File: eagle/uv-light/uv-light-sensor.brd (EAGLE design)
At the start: 17 x 13 mm, 4 parts, among them IC100 SI1147

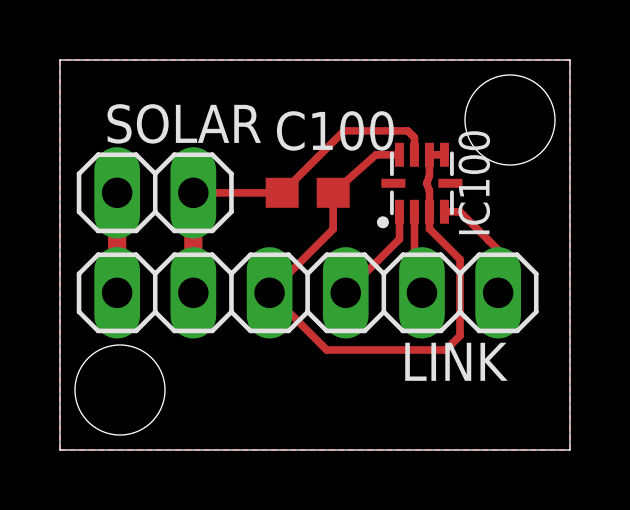
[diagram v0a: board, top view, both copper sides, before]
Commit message: CHG: updated lib, schematics and boards
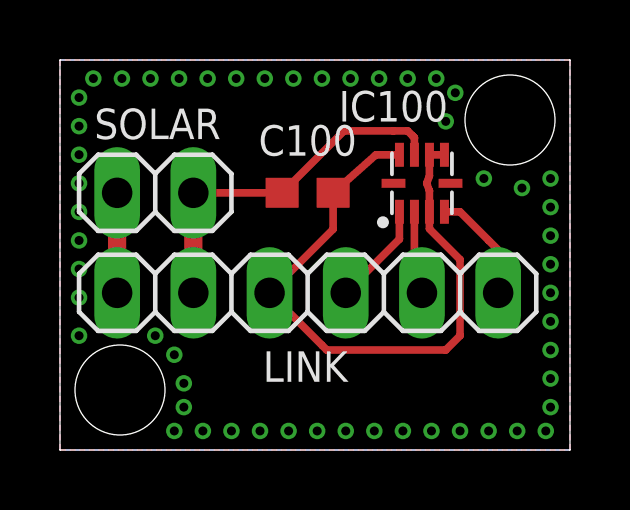
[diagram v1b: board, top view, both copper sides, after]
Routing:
- net GND: vias 0 -> 53
- added copper zone on layer 16, net GND
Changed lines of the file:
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@@
 <element name="IC100" library="weather_station" package="QFN-10/2MM" value="SI1147" x="12.065" y="8.89" smashed="yes" rot="R90">
 <attribute name="DIGIKEY" value="336-2624-1-ND" x="26.035" y="24.13" size="1.778" layer="27" rot="R90" display="off"/>
-<attribute name="NAME" x="14.31625" y="8.89" size="1.016" layer="25" font="vector" ratio="12" rot="R90" align="bottom-center"/>
+<attribute name="NAME" x="11.1125" y="11.45875" size="1.016" layer="25" font="vector" ratio="12" rot="R180" align="center"/>
 </element>
 <element name="C100" library="rcl" package="C0603" value="100n" x="8.255" y="8.5725" smashed="yes">
-<attribute name="NAME" x="7.14375" y="10.00125" size="1.27" layer="25"/>
+<attribute name="NAME" x="8.255" y="10.31875" size="1.016" layer="25" align="center"/>
 <attribute name="VALUE" x="7.62" y="6.6675" size="1.27" layer="27"/>
 </element>
 <element name="LINK" library="pinhead" package="1X06" value="" x="8.255" y="5.23875" smashed="yes">
-<attribute name="NAME" x="11.3538" y="2.30505" size="1.27" layer="25" ratio="10"/>
+<attribute name="NAME" x="8.1788" y="2.7813" size="1.016" layer="25" ratio="10" align="center"/>
 <attribute name="VALUE" x="0.635" y="2.06375" size="1.27" layer="27"/>
 </element>
 <element name="SOLAR" library="pinhead" package="1X02" value="" x="3.175" y="8.5725" smashed="yes" rot="R180">
-<attribute name="NAME" x="6.7437" y="11.5062" size="1.27" layer="25" ratio="10" rot="R180"/>
+<attribute name="NAME" x="3.2512" y="10.8712" size="1.016" layer="25" ratio="10" rot="R180" align="center"/>
 <attribute name="VALUE" x="5.715" y="11.7475" size="1.27" layer="27" rot="R180"/>
 </element>
@@
 <wire x1="11.7475" y1="10.4775" x2="11.815" y2="10.41" width="0.254" layer="1"/>
 <wire x1="11.815" y1="10.41" x2="11.815" y2="9.84" width="0.254" layer="1"/>
-<polygon width="0.4064" layer="1" thermals="no">
+<polygon width="0.3048" layer="1" thermals="no">
 <vertex x="0" y="13"/>
 <vertex x="0" y="0"/>
@@
 <vertex x="17" y="13"/>
 </polygon>
+<via x="3.81" y="0.635" extent="1-16" drill="0.3"/>
+<polygon width="0.3048" layer="16" thermals="no">
+<vertex x="0" y="13"/>
+<vertex x="17" y="13"/>
+<vertex x="17" y="0"/>
+<vertex x="0" y="0"/>
+</polygon>
+<via x="4.7625" y="0.635" extent="1-16" drill="0.3"/>
+<via x="5.715" y="0.635" extent="1-16" drill="0.3"/>
+<via x="6.6675" y="0.635" extent="1-16" drill="0.3"/>
+<via x="7.62" y="0.635" extent="1-16" drill="0.3"/>
+<via x="8.5725" y="0.635" extent="1-16" drill="0.3"/>
+<via x="9.525" y="0.635" extent="1-16" drill="0.3"/>
+<via x="10.4775" y="0.635" extent="1-16" drill="0.3"/>
+<via x="11.43" y="0.635" extent="1-16" drill="0.3"/>
+<via x="12.3825" y="0.635" extent="1-16" drill="0.3"/>
+<via x="13.335" y="0.635" extent="1-16" drill="0.3"/>
+<via x="14.2875" y="0.635" extent="1-16" drill="0.3"/>
+<via x="15.24" y="0.635" extent="1-16" drill="0.3"/>
+<via x="16.1925" y="0.635" extent="1-16" drill="0.3"/>
+<via x="16.35125" y="1.42875" extent="1-16" drill="0.3"/>
+<via x="16.35125" y="2.38125" extent="1-16" drill="0.3"/>
+<via x="16.35125" y="3.33375" extent="1-16" drill="0.3"/>
+<via x="16.35125" y="4.28625" extent="1-16" drill="0.3"/>
+<via x="16.35125" y="5.23875" extent="1-16" drill="0.3"/>
+<via x="16.35125" y="6.19125" extent="1-16" drill="0.3"/>
+<via x="16.35125" y="7.14375" extent="1-16" drill="0.3"/>
+<via x="16.35125" y="8.09625" extent="1-16" drill="0.3"/>
+<via x="16.35125" y="9.04875" extent="1-16" drill="0.3"/>
+<via x="15.39875" y="8.73125" extent="1-16" drill="0.3"/>
+<via x="14.12875" y="9.04875" extent="1-16" drill="0.3"/>
+<via x="12.85875" y="10.95375" extent="1-16" drill="0.3"/>
+<via x="13.17625" y="11.90625" extent="1-16" drill="0.3"/>
+<via x="12.54125" y="12.3825" extent="1-16" drill="0.3"/>
+<via x="11.58875" y="12.3825" extent="1-16" drill="0.3"/>
+<via x="10.63625" y="12.3825" extent="1-16" drill="0.3"/>
+<via x="9.68375" y="12.3825" extent="1-16" drill="0.3"/>
+<via x="8.73125" y="12.3825" extent="1-16" drill="0.3"/>
+<via x="7.77875" y="12.3825" extent="1-16" drill="0.3"/>
+<via x="6.82625" y="12.3825" extent="1-16" drill="0.3"/>
+<via x="5.87375" y="12.3825" extent="1-16" drill="0.3"/>
+<via x="4.92125" y="12.3825" extent="1-16" drill="0.3"/>
+<via x="3.96875" y="12.3825" extent="1-16" drill="0.3"/>
+<via x="3.01625" y="12.3825" extent="1-16" drill="0.3"/>
+<via x="2.06375" y="12.3825" extent="1-16" drill="0.3"/>
+<via x="1.11125" y="12.3825" extent="1-16" drill="0.3"/>
+<via x="0.635" y="11.7475" extent="1-16" drill="0.3"/>
+<via x="0.635" y="10.795" extent="1-16" drill="0.3"/>
+<via x="0.635" y="9.8425" extent="1-16" drill="0.3"/>
+<via x="0.635" y="8.89" extent="1-16" drill="0.3"/>
+<via x="0.635" y="7.9375" extent="1-16" drill="0.3"/>
+<via x="0.635" y="6.985" extent="1-16" drill="0.3"/>
+<via x="0.635" y="6.0325" extent="1-16" drill="0.3"/>
+<via x="0.635" y="5.08" extent="1-16" drill="0.3"/>
+<via x="0.635" y="3.81" extent="1-16" drill="0.3"/>
+<via x="3.175" y="3.81" extent="1-16" drill="0.3"/>
+<via x="3.81" y="3.175" extent="1-16" drill="0.3"/>
+<via x="4.1275" y="2.2225" extent="1-16" drill="0.3"/>
+<via x="4.1275" y="1.42875" extent="1-16" drill="0.3"/>
 </signal>
 <signal name="N$1">
